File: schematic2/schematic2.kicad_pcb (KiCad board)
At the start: 2 copper layers, 68.8 x 56 mm, 48 parts, among them K1 TIANBO_HJR_1-2C, P1 Conn_02x20_Odd_Even, Q1 BC547, Q2 2N2907, Q3 BC547, Q4 BC547, U1 AP1117-33, U1 buck, U2 DS3231M, U4 CAT24C256

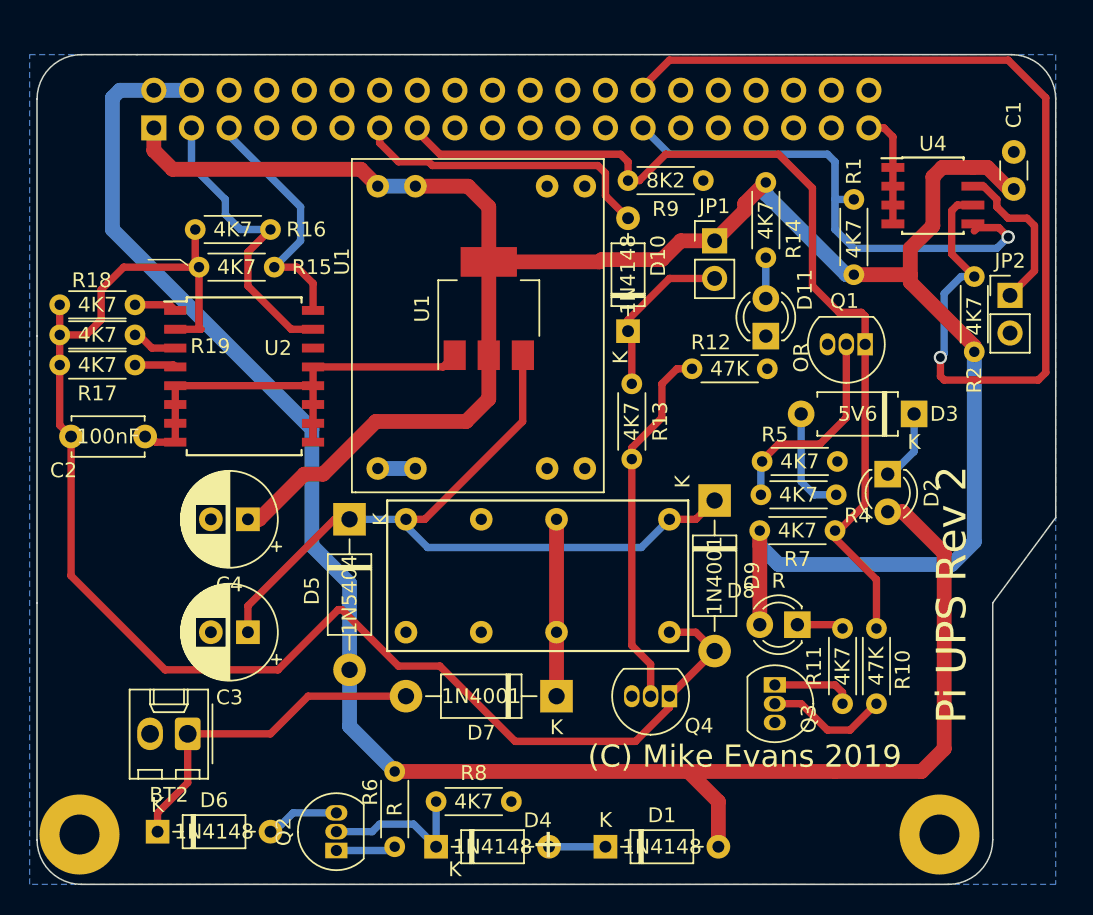
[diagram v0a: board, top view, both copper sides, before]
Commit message: modified:   doc/UPS.adoc modified:   firmware/src/powermon.py modified:   schematic2/schematic2-cache.lib modified:   schematic2/schematic2.kicad_pcb modified:   schematic2/schematic2.sch
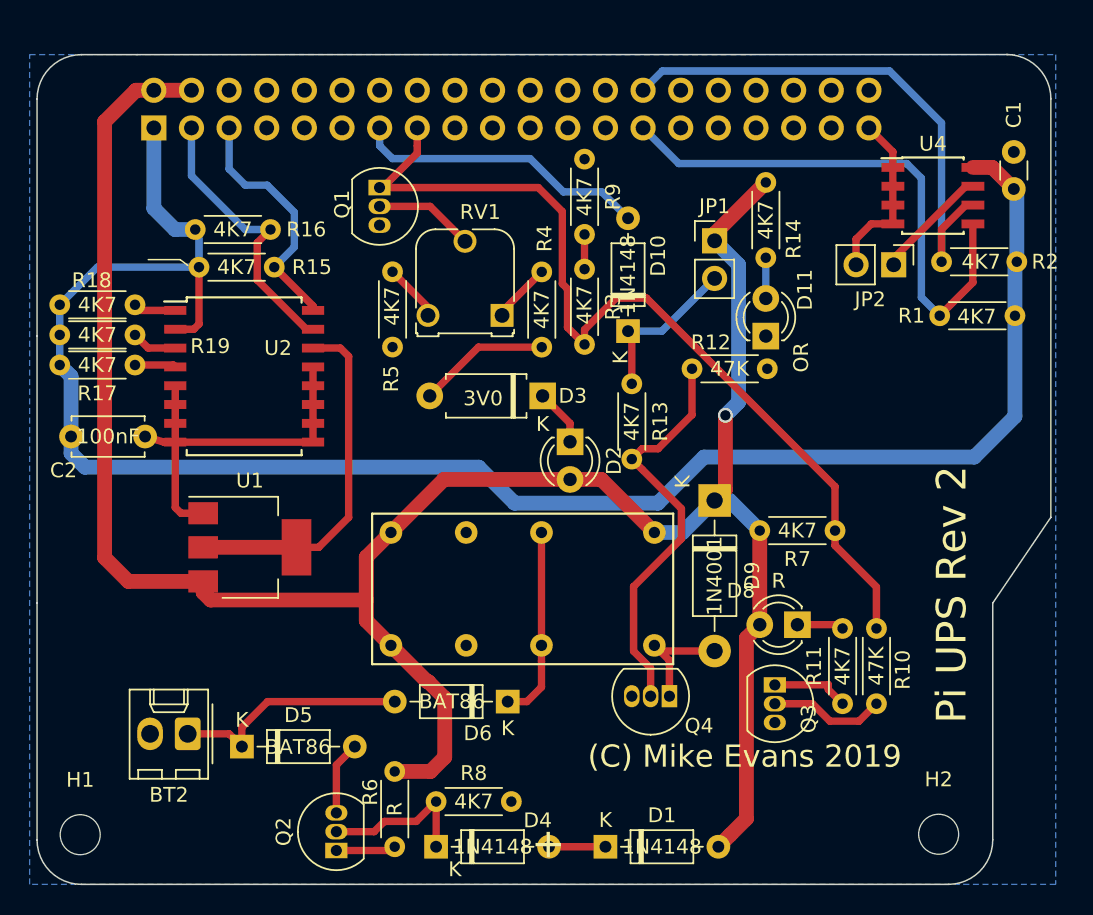
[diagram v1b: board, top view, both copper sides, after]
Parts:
- removed C3: 10uF, Capacitor_THT:CP_Radial_D6.3mm_P2.50mm
- removed C4: 22uF, Capacitor_THT:CP_Radial_D6.3mm_P2.50mm
- removed D7: 1N4001, Diode_THT:D_DO-41_SOD81_P10.16mm_Horizontal
- removed REF** (x2): MountingHole_2.7mm_M2.5_Pad, MountingHole:MountingHole_2.7mm_M2.5_Pad
- removed the U1 at (231.0, 111.1)
- removed the U1 at (231.8, 113.0)
- added H1: MountingHole, MountingHole:MountingHole_2.7mm, F.Cu at (203.4, 146.6)
- added H2: MountingHole, MountingHole:MountingHole_2.7mm, F.Cu at (261.3, 146.6)
- added R3: 4K7, Resistor_THT:R_Axial_DIN0204_L3.6mm_D1.6mm_P5.08mm_Horizontal, F.Cu at (237.4, 108.5)
- added RV1: R_POT_TRIM, Potentiometer_THT:Potentiometer_Runtron_RM-065_Vertical, F.Cu at (231.9, 111.6)
- added U1: AP1117-33, Package_TO_SOT_SMD:SOT-223-3_TabPin2, F.Cu at (214.9, 127.3)
- D3: value 5V6 -> 3V0
- D5: value 1N5404 -> BAT86; footprint Diode_THT:D_DO-41_SOD81_P10.16mm_Horizontal -> Diode_THT:D_DO-35_SOD27_P7.62mm_Horizontal
- D6: value 1N4148 -> BAT86
- R9: value 8K2 -> 4K7
- moved Q1 34.4 mm to (223.6, 103.0), turned to 270 degrees
- moved R5 28.0 mm to (224.5, 108.7), turned to 270 degrees
- moved D6 25.2 mm to (232.3, 137.7), turned to 180 degrees
- moved D3 25.1 mm to (234.6, 117.0)
- moved R4 22.2 mm to (234.6, 113.7), turned to 90 degrees
- moved D2 21.6 mm to (236.5, 120.1)
- moved D5 17.0 mm to (214.3, 140.7), turned to 0 degrees
- moved R1 11.2 mm to (266.5, 111.6), turned to 180 degrees
- moved R9 8.15 mm to (237.4, 101.1), turned to 270 degrees
- moved JP2 8.12 mm to (258.3, 108.2), turned to 270 degrees
- moved R2 6.72 mm to (266.6, 108.0), turned to 180 degrees
- moved K1 1.35 mm to (242.2, 133.9)
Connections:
- C2 pad 1: /Sheet5B4BA297/VI -> +3V3
- D10 pad 1: Net-(D10-Pad1) -> +5V
- D5 pad 1: Net-(C3-Pad1) -> Net-(BT2-Pad1)
- D5 pad 2: +5V -> Net-(D5-Pad2)
- D6 pad 1: Net-(BT2-Pad1) -> Net-(D6-Pad1)
- D6 pad 2: Net-(D6-Pad2) -> Net-(BT2-Pad1)
- D8 pad 2: +3V3 -> +5V
- D9 pad 1: Net-(C3-Pad1) -> +5V
- D9 pad 2: /Sheet5B4BA297/VI -> Net-(D9-Pad2)
- JP1 pad 1: +3V3 -> +5V
- JP1 pad 2: Net-(D10-Pad1) -> (no net)
- K1 pad 1: /Sheet5B4BA297/VI -> Net-(D9-Pad2)
- K1 pad 13: Net-(D7-Pad1) -> Net-(D6-Pad1)
- K1 pad 16: Net-(C3-Pad1) -> +5V
- K1 pad 4: Net-(D7-Pad1) -> Net-(D6-Pad1)
- K1 pad 8: (no net) -> +5V
- K1 pad 9: Net-(C3-Pad1) -> +5V
- Q2 pad 3: Net-(D6-Pad2) -> Net-(D5-Pad2)
- Q4 pad 1: /Sheet5B4BA297/VI -> Net-(D9-Pad2)
- R13 pad 1: Net-(D10-Pad1) -> +5V
- R14 pad 2: +3V3 -> +5V
- R15 pad 2: /Sheet5B4BA297/VI -> +3V3
- R16 pad 2: /Sheet5B4BA297/VI -> +3V3
- R17 pad 2: /Sheet5B4BA297/VI -> +3V3
- R18 pad 2: /Sheet5B4BA297/VI -> +3V3
- R19 pad 2: /Sheet5B4BA297/VI -> +3V3
- R4 pad 2: Net-(Q1-Pad2) -> Net-(R4-Pad2)
- R5 pad 1: Net-(Q1-Pad2) -> Net-(R5-Pad1)
- R7 pad 2: +3V3 -> +5V
- R9 pad 2: POWER_FAIL -> Net-(R3-Pad1)
- U2 pad 14: (no net) -> V_BAT
- U2 pad 2: /Sheet5B4BA297/VI -> +3V3
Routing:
- net /Sheet5B4BA297/VI: track 97.7 -> 0.00 mm
- net Net-(C3-Pad1): track 53.1 -> 0.00 mm
- net +5V: track 120.7 -> 164.6 mm, vias 0 -> 1
- net ID_SC: track 70.3 -> 36.5 mm, vias 1 -> 0
- net +3V3: track 148.8 -> 124.2 mm
- net V_BAT: track 0.00 -> 24.2 mm
- net Net-(D6-Pad1): track 0.00 -> 13.1 mm
- net Net-(D7-Pad1): track 11.9 -> 0.00 mm
- net Net-(D10-Pad1): track 11.4 -> 0.00 mm
- net Net-(D9-Pad2): track 0.00 -> 8.07 mm
- net Net-(Q1-Pad2): track 14.2 -> 6.75 mm
- net Net-(BT2-Pad1): track 23.2 -> 16.4 mm
- net Net-(D5-Pad2): track 0.00 -> 4.99 mm
- net Net-(D6-Pad2): track 4.97 -> 0.00 mm
- net Net-(R4-Pad2): track 0.00 -> 3.67 mm
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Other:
- board size 68.8 x 56 mm -> 68.4 x 56 mm
- board text removed: "BOTOM LEGEND"
- board text removed: "BOTTOM ASSEMBLY"
- board text removed: "TOP ASSEMBLY"
- board text removed: "TOP LEGEND"

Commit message: Mostly layout changes.
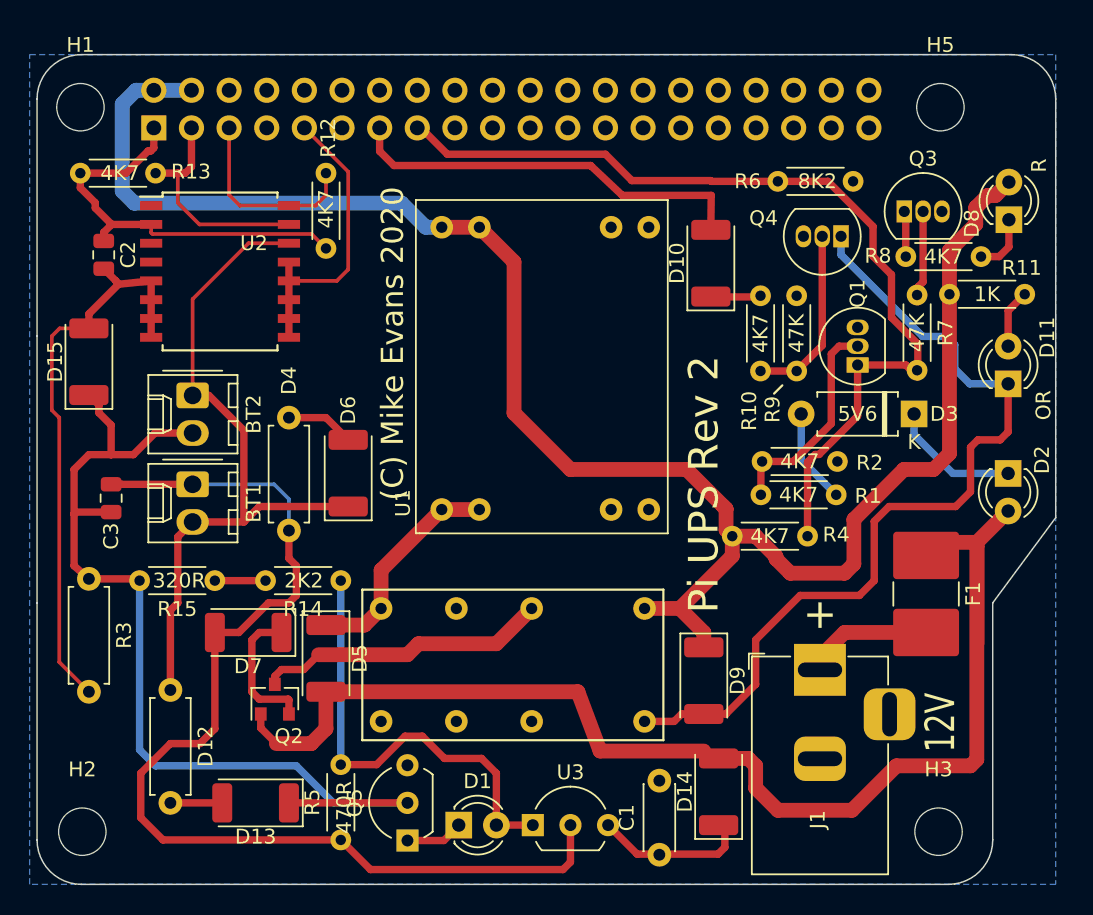
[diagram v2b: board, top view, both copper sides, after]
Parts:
- removed JP1: UPS, Connector_PinHeader_2.54mm:PinHeader_1x02_P2.54mm_Vertical
- removed JP2: Jumper_NO_Small, Connector_PinHeader_2.54mm:PinHeader_1x02_P2.54mm_Vertical
- removed the R1 at (266.5, 111.6)
- removed the R10 at (257.1, 137.8)
- removed R16, R17, R18, R19: 4K7, Resistor_THT:R_Axial_DIN0204_L3.6mm_D1.6mm_P5.08mm_Horizontal
- removed the R2 at (266.6, 108.0)
- removed the R6 at (224.6, 147.5)
- removed the R8 at (227.4, 144.4)
- removed RV1: R_POT_TRIM, Potentiometer_THT:Potentiometer_Runtron_RM-065_Vertical
- removed U4: CAT24C256, Package_SO:SOIC-8_3.9x4.9mm_P1.27mm
- added BT1: Battery_Cell, Connector_Molex:Molex_KK-254_AE-6410-02A_1x02_P2.54mm_Vertical, F.Cu at (211.0, 123.0)
- added C3: 100n, Capacitor_SMD:C_0805_2012Metric, F.Cu at (205.5, 123.9)
- added D12: 3V6, Resistor_THT:R_Axial_DIN0207_L6.3mm_D2.5mm_P7.62mm_Horizontal, F.Cu at (209.5, 136.9)
- added D13: 1N4001, Diode_SMD:D_2010_5025Metric, F.Cu at (215.2, 144.5)
- added D14: 1N4001, Diode_SMD:D_2010_5025Metric, F.Cu at (246.5, 143.8)
- added D15: 1N4001, Diode_SMD:D_2010_5025Metric, F.Cu at (204.0, 114.7)
- added D7: 1N4001, Diode_SMD:D_2010_5025Metric, F.Cu at (214.8, 133.0)
- added F1: Polyfuse, Fuse:Fuse_2816_7142Metric_Pad3.20x4.45mm_HandSolder, F.Cu at (260.5, 130.4)
- added H3: MountingHole, MountingHole:MountingHole_3.2mm_M3, F.Cu at (261.3, 146.4)
- added H5: MountingHole, MountingHole:MountingHole_3.2mm_M3, F.Cu at (261.5, 97.5)
- added J1: Barrel_Jack, Connector_BarrelJack:BarrelJack_Horizontal, F.Cu at (253.3, 135.5)
- added Q5: BC547, Package_TO_SOT_THT:TO-92L_Inline_Wide, F.Cu at (225.5, 147.0)
- added R12: 4K7, Resistor_THT:R_Axial_DIN0204_L3.6mm_D1.6mm_P5.08mm_Horizontal, F.Cu at (220.0, 102.0)
- added R13: 4K7, Resistor_THT:R_Axial_DIN0204_L3.6mm_D1.6mm_P5.08mm_Horizontal, F.Cu at (208.5, 102.0)
- added R14: 2K2, Resistor_THT:R_Axial_DIN0204_L3.6mm_D1.6mm_P5.08mm_Horizontal, F.Cu at (221.0, 129.5)
- added R5: 470R, Resistor_THT:R_Axial_DIN0204_L3.6mm_D1.6mm_P5.08mm_Horizontal, F.Cu at (221.0, 147.0)
- added R7: 47K, Resistor_THT:R_Axial_DIN0204_L3.6mm_D1.6mm_P5.08mm_Horizontal, F.Cu at (259.9, 110.2)
- added U3: LM317_SOT-223, Package_TO_SOT_THT:TO-92L_Inline_Wide, F.Cu at (234.0, 146.0)
- BT2: value 4x AAA NiMh -> Battery_Cell
- C1: value C_Small -> 100n; footprint Capacitor_THT:C_Disc_D3.0mm_W1.6mm_P2.50mm -> Capacitor_THT:C_Disc_D4.3mm_W1.9mm_P5.00mm
- C2: footprint Capacitor_THT:C_Disc_D4.7mm_W2.5mm_P5.00mm -> Capacitor_SMD:C_0805_2012Metric
- D1: value 1N4148 -> LED; footprint Diode_THT:D_DO-35_SOD27_P7.62mm_Horizontal -> LED_THT:LED_D3.0mm
- D10: footprint Diode_THT:D_DO-35_SOD27_P7.62mm_Horizontal -> Diode_SMD:D_2010_5025Metric
- D3: value 3V0 -> 5V6
- D4: value 1N4148 -> 3V6; footprint Diode_THT:D_DO-35_SOD27_P7.62mm_Horizontal -> Resistor_THT:R_Axial_DIN0207_L6.3mm_D2.5mm_P7.62mm_Horizontal
- D5, D6: value BAT86 -> 1N4001; footprint Diode_THT:D_DO-35_SOD27_P7.62mm_Horizontal -> Diode_SMD:D_2010_5025Metric
- D9: footprint Diode_THT:D_DO-41_SOD81_P10.16mm_Horizontal -> Diode_SMD:D_2010_5025Metric
- H1, H2: footprint MountingHole:MountingHole_2.7mm -> MountingHole:MountingHole_3.2mm_M3
- Q2: value 2N2907 -> DMP1045U; footprint Package_TO_SOT_THT:TO-92_Inline -> Package_TO_SOT_SMD:SOT-23
- R11: renamed from R14; value 4K7 -> 1K
- R15: value 4K7 -> 320R
- R3: value 4K7 -> 6R6; footprint Resistor_THT:R_Axial_DIN0204_L3.6mm_D1.6mm_P5.08mm_Horizontal -> Resistor_THT:R_Axial_DIN0207_L6.3mm_D2.5mm_P7.62mm_Horizontal
- R6: renamed from R9; value 4K7 -> 8K2
- U1: value AP1117-33 -> buck; footprint Package_TO_SOT_SMD:SOT-223-3_TabPin2 -> Mikee:BUCK_MODULE_5V
- moved H2 57.8 mm to (203.6, 146.4)
- moved C1 50.9 mm to (242.5, 148.0)
- moved H1 49.1 mm to (203.4, 97.5)
- moved R3 39.4 mm to (204.0, 129.4)
- moved Q1 34.4 mm to (255.9, 114.9), turned to 90 degrees
- moved Q4 33.1 mm to (254.8, 106.3)
- moved Q3 33.1 mm to (259.0, 104.6), turned to 0 degrees
- moved D8 30.8 mm to (266.1, 105.1), turned to 90 degrees
- moved R8 30.5 mm to (259.1, 107.6), turned to 0 degrees
- moved D2 29.6 mm to (266.0, 122.3)
- moved R2 28.0 mm to (249.4, 121.5), turned to 0 degrees
- moved D3 25.1 mm to (259.7, 118.2)
- moved U1 24.1 mm to (236.1, 115.8), turned to 90 degrees
- moved D4 23.5 mm to (217.5, 126.1), turned to 90 degrees
- moved BT2 22.8 mm to (211.0, 117.0), turned to 270 degrees
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- renumbered R4 to R1, R13 to R10, R5 to R2, R7 to R4, R11 to R8, R12 to R9
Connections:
- BT2 pad 1: Net-(BT2-Pad1) -> CLK_BAT
- BT2 pad 2: GND -> Net-(BT2-Pad2)
- C1 pad 1: +3V3 -> Net-(C1-Pad1)
- D1 pad 2: +5V -> Net-(D1-Pad2)
- D10 pad 1: +5V -> Net-(D10-Pad1)
- D11 pad 1: GND -> Net-(D11-Pad1)
- D2 pad 2: +5V -> +9V
- D4 pad 1: Net-(D4-Pad1) -> Net-(BT1-Pad1)
- D4 pad 2: Net-(D1-Pad1) -> Net-(D4-Pad2)
- D5 pad 1: Net-(BT2-Pad1) -> Net-(D5-Pad1)
- D5 pad 2: Net-(D5-Pad2) -> +9V
- D6 pad 1: Net-(D6-Pad1) -> CLK_BAT
- D6 pad 2: Net-(BT2-Pad1) -> Net-(D4-Pad2)
- D9 pad 2: Net-(D9-Pad2) -> Net-(D11-Pad1)
- K1 pad 1: Net-(D9-Pad2) -> Net-(D11-Pad1)
- K1 pad 13: Net-(D6-Pad1) -> Net-(K1-Pad13)
- K1 pad 4: Net-(D6-Pad1) -> (no net)
- K1 pad 8: +5V -> (no net)
- K1 pad 9: +5V -> Net-(D5-Pad1)
- P1 pad 27: ID_SD -> (no net)
- P1 pad 28: ID_SC -> (no net)
- Q2 pad 1: Net-(Q2-Pad1) -> +9V
- Q2 pad 2: Net-(D4-Pad1) -> Net-(D7-Pad1)
- Q2 pad 3: Net-(D5-Pad2) -> Net-(K1-Pad13)
- Q4 pad 1: Net-(D9-Pad2) -> Net-(D11-Pad1)
- R1 pad 2: Net-(R4-Pad2) -> Net-(Q1-Pad2)
- R10 pad 1: +5V -> Net-(D10-Pad1)
- R15 pad 1: SCL1 -> Net-(R14-Pad2)
- R15 pad 2: +3V3 -> Net-(BT2-Pad2)
- R2 pad 1: Net-(R5-Pad1) -> Net-(Q1-Pad2)
- R3 pad 1: Net-(R3-Pad1) -> Net-(BT2-Pad2)
- R3 pad 2: POWER_FAIL -> GND
- R6 pad 2: Net-(R3-Pad1) -> POWER_FAIL
- U1 pad 1: GND -> Net-(D5-Pad1)
- U1 pad 2: V_BAT -> GND
- U1 pad 3: +5V -> GND
- U2 pad 1: Net-(R18-Pad1) -> (no net)
- U2 pad 14: V_BAT -> CLK_BAT
- U2 pad 3: Net-(R19-Pad1) -> (no net)
- U2 pad 4: Net-(R17-Pad1) -> (no net)
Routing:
- net +3V3: track 124.2 -> 28.2 mm
- net +9V: track 0.00 -> 87.4 mm
- net Net-(BT1-Pad1): track 0.00 -> 74.6 mm
- net Net-(BT2-Pad2): track 0.00 -> 66.5 mm
- net Net-(D11-Pad1): track 0.00 -> 59.3 mm
- net CLK_BAT: track 0.00 -> 48.1 mm
- net +5V: track 164.6 -> 122.1 mm, vias 1 -> 0
- net ID_SD: track 37.1 -> 0.00 mm
- net ID_SC: track 36.5 -> 0.00 mm
- net Net-(D1-Pad2): track 0.00 -> 30.7 mm
- net V_BAT: track 24.2 -> 0.00 mm
- net GND: track 38.5 -> 59.2 mm
- net Net-(K1-Pad13): track 0.00 -> 19.8 mm
- net Net-(BT2-Pad1): track 16.4 -> 0.00 mm
- net Net-(Q4-Pad2): track 27.6 -> 12.2 mm
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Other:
- board size 68.4 x 56 mm -> 68.8 x 56 mm
- net class Bat_Charge added: clearance 0.1, trace_width 0.25, via_dia 0.9, via_drill 0.6
- board text added: "(C) Mike Evans 2020"
- board text added: "12V"
- board text removed: "(C) Mike Evans 2019"
- board text removed: "A/V"
- board text removed: "ACT"
- board text removed: "C1"
- board text removed: "C10"
- board text removed: "C101"
- board text removed: "C102"
- board text removed: "C103"
- board text removed: "C106"
- board text removed: "C11"
- board text removed: "C14"
- board text removed: "C162"
- board text removed: "C163"
- board text removed: "C165"
- board text removed: "C187"
- board text removed: "C188"
- board text removed: "C190"
- board text removed: "C192"
- board text removed: "C194"
- board text removed: "C2"
- board text removed: "C200"
- board text removed: "C201"
- board text removed: "C204"
- board text removed: "C210"
- board text removed: "C211"
- board text removed: "C212"
- board text removed: "C213"
- board text removed: "C214"
- board text removed: "C215"
- board text removed: "C216"
- board text removed: "C217"
- board text removed: "C218"
- board text removed: "C219"
- board text removed: "C220"
- board text removed: "C221"
- board text removed: "C222"
- board text removed: "C224"
- board text removed: "C226"
- board text removed: "C227"
- board text removed: "C228"
- board text removed: "C229"
- board text removed: "C230"
- board text removed: "C231"
- board text removed: "C233"
- board text removed: "C235"
- board text removed: "C237"
- board text removed: "C238"
- board text removed: "C239"
- board text removed: "C240"
- board text removed: "C241"
- board text removed: "C243"
- board text removed: "C245"
- board text removed: "C246"
- board text removed: "C248"
- board text removed: "C252"
- board text removed: "C255"
- board text removed: "C256"
- board text removed: "C258"
- board text removed: "C259"
- board text removed: "C3"
- board text removed: "C4"
- board text removed: "C46"
- board text removed: "C47"
- board text removed: "C48"
- board text removed: "C5"
- board text removed: "C52"
- board text removed: "C53"
- board text removed: "C54"
- board text removed: "C55"
- board text removed: "C56"
- board text removed: "C57"
- board text removed: "C58"
- board text removed: "C59"
- board text removed: "C6"
- board text removed: "C60"
- board text removed: "C61"
- board text removed: "C62"
- board text removed: "C63"
- board text removed: "C64"
- board text removed: "C65"
- board text removed: "C66"
- board text removed: "C67"
- board text removed: "C7"
- board text removed: "C70"
- board text removed: "C71"
- board text removed: "C72"
- board text removed: "C73"
- board text removed: "C74"
- board text removed: "C75"
- board text removed: "C76"
- board text removed: "C77"
- board text removed: "C78"
- board text removed: "C79"
- board text removed: "C8"
- board text removed: "C80"
- board text removed: "C81"
- board text removed: "C82"
- board text removed: "C83"
- board text removed: "C84"
- board text removed: "C85"
- board text removed: "C86"
- board text removed: "C87"
- board text removed: "C88"
- board text removed: "C89"
- board text removed: "C90"
- board text removed: "C91"
- board text removed: "C92"
- board text removed: "C93"
- board text removed: "C94"
- board text removed: "C96"
- board text removed: "C97"
- board text removed: "C98"
- board text removed: "C99"
- board text removed: "CAMERA"
- board text removed: "D3"
- board text removed: "D4"
- board text removed: "D5"
- board text removed: "DISPLAY"
- board text removed: "ETHERNET"
- board text removed: "F1"
- board text removed: "FB1"
- board text removed: "FB2"
- board text removed: "FB3"
- board text removed: "FB4"
- board text removed: "FB5"
- board text removed: "FB6"
- board text removed: "FB7"
- board text removed: "FB8"
- board text removed: "FCC ID: 2ABCB-RPI32"
- board text removed: "GPIO"
- board text removed: "HDMI"
- board text removed: "IC: 20953-RPI32"
- board text removed: "J1"
- board text removed: "J10"
- board text removed: "J11"
- board text removed: "J12"
- board text removed: "J13"
- board text removed: "J3"
- board text removed: "J4"
- board text removed: "J5"
- board text removed: "J6"
- board text removed: "J7"
- board text removed: "J8"
- board text removed: "J9"
- board text removed: "L1"
- board text removed: "L2"
- board text removed: "L3"
- board text removed: "L4"
- board text removed: "L5"
- board text removed: "L6"
- board text removed: "L7"
- board text removed: "L8"
- board text removed: "MICRO SD CARD"
- board text removed: "Made in the UK"
- board text removed: "PP1"
- board text removed: "PP10"
- board text removed: "PP11"
- board text removed: "PP12"
- board text removed: "PP13"
- board text removed: "PP2"
- board text removed: "PP20"
- board text removed: "PP21"
- board text removed: "PP22"
- board text removed: "PP23"
- board text removed: "PP24"
- board text removed: "PP25"
- board text removed: "PP26"
- board text removed: "PP27"
- board text removed: "PP28"
- board text removed: "PP3"
- board text removed: "PP35"
- board text removed: "PP36"
- board text removed: "PP39"
- board text removed: "PP4"
- board text removed: "PP40"
- board text removed: "PP41"
- board text removed: "PP42"
- board text removed: "PP43"
- board text removed: "PP44"
- board text removed: "PP45"
- board text removed: "PP46"
- board text removed: "PP47"
- board text removed: "PP48"
- board text removed: "PP49"
- board text removed: "PP5"
- board text removed: "PP50"
- board text removed: "PP51"
- board text removed: "PP52"
- board text removed: "PP53"
- board text removed: "PP54"
- board text removed: "PP55"
- board text removed: "PP56"
- board text removed: "PP57"
- board text removed: "PP58"
- board text removed: "PP59"
- board text removed: "PP6"
- board text removed: "PP60"
- board text removed: "PP7"
- board text removed: "PP8"
- board text removed: "PP9"
- board text removed: "PWR"
- board text removed: "PWR IN"
- board text removed: "Q1"
- board text removed: "Q2"
- board text removed: "Q3"
- board text removed: "Q4"
- board text removed: "Q5"
- board text removed: "Q6"
- board text removed: "Q7"
- board text removed: "Q8"
- board text removed: "R1"
- board text removed: "R10"
- board text removed: "R12"
- board text removed: "R13"
- board text removed: "R14"
- board text removed: "R15"
- board text removed: "R16"
- board text removed: "R17"
- board text removed: "R18"
- board text removed: "R19"
- board text removed: "R2"
- board text removed: "R20"
- board text removed: "R21"
- board text removed: "R22"
- board text removed: "R23"
- board text removed: "R24"
- board text removed: "R25"
- board text removed: "R3"
- board text removed: "R31"
- board text removed: "R32"
- board text removed: "R33"
- board text removed: "R34"
- board text removed: "R35"
- board text removed: "R36"
- board text removed: "R37"
- board text removed: "R38"
- board text removed: "R39"
- board text removed: "R4"
- board text removed: "R41"
- board text removed: "R42"
- board text removed: "R43"
- board text removed: "R44"
- board text removed: "R45"
- board text removed: "R46"
- board text removed: "R47"
- board text removed: "R48"
- board text removed: "R5"
- board text removed: "R50"
- board text removed: "R51"
- board text removed: "R52"
- board text removed: "R54"
- board text removed: "R55"
- board text removed: "R56"
- board text removed: "R57"
- board text removed: "R58"
- board text removed: "R6"
- board text removed: "R60"
- board text removed: "R61"
- board text removed: "R63"
- board text removed: "R64"
- board text removed: "R65"
- board text removed: "R66"
- board text removed: "R67"
- board text removed: "R68"
- board text removed: "R69"
- board text removed: "R7"
- board text removed: "R70"
- board text removed: "R71"
- board text removed: "R72"
- board text removed: "R75"
- board text removed: "R76"
- board text removed: "R77"
- board text removed: "R78"
- board text removed: "R79"
- board text removed: "R8"
- board text removed: "R81"
- board text removed: "R82"
- board text removed: "R83"
- board text removed: "RUN"
- board text removed: "Raspberry Pi 3 Model B V1.2"
- board text removed: "U1"
- board text removed: "U10"
- board text removed: "U11"
- board text removed: "U13"
- board text removed: "U14"
- board text removed: "U15"
- board text removed: "U16"
- board text removed: "U17"
- board text removed: "U18"
- board text removed: "U19"
- board text removed: "U2"
- board text removed: "U20"
- board text removed: "U3"
- board text removed: "U4"
- board text removed: "U5"
- board text removed: "U8"
- board text removed: "U9"
- board text removed: "X1"
- board text removed: "X2"
- board text removed: "c Raspberry Pi 2015"
